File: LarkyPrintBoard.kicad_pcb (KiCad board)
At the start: 2 copper layers, 38 x 56 mm, 27 parts, among them J1 EXT1_IN, J2 EXT2_IN, J3 EXT1_OUT, J4 EXT2_OUT, J5 UART, J6 RST, J7 BOOT, J8 3V3, J9 JTAG, U1 LM1117-3.3, U2 ESP32-WROOM, U3 CBT3257A, U4 CBT3257A

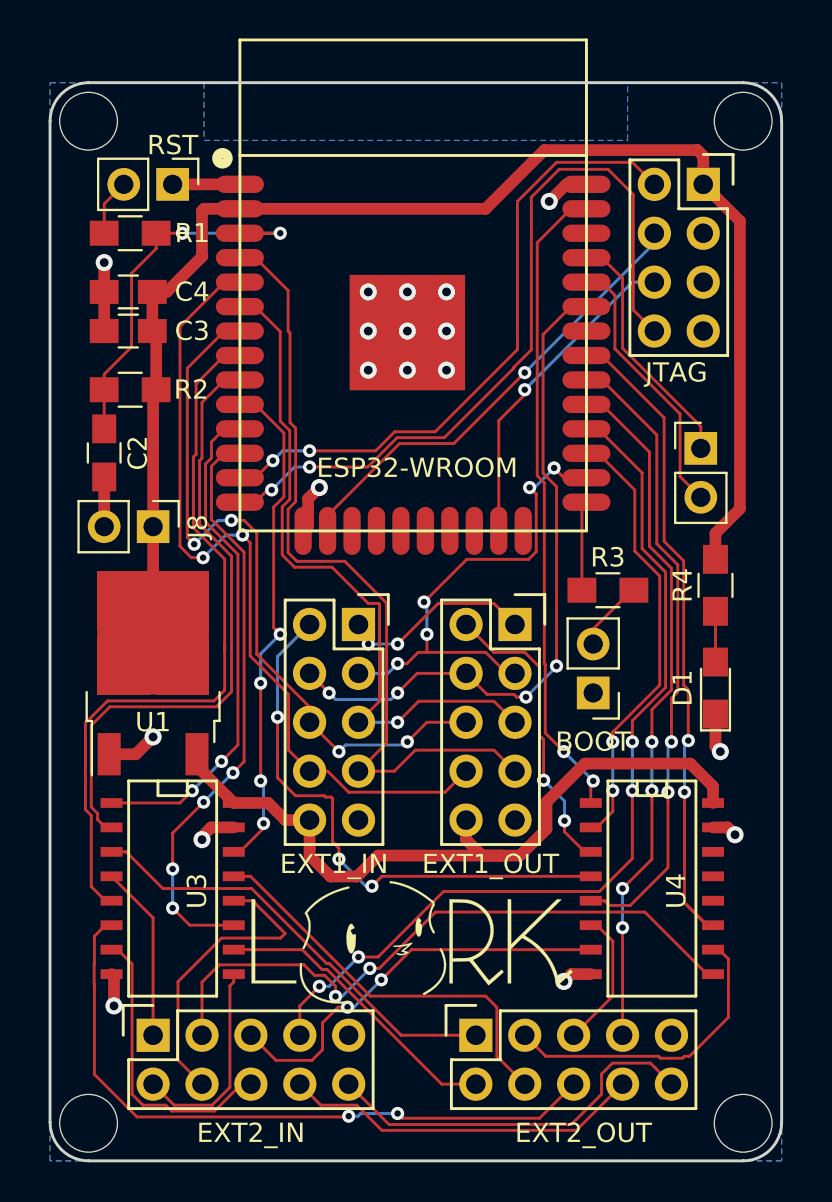
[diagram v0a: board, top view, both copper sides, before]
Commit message: Tons of changes and fixes. R1A2
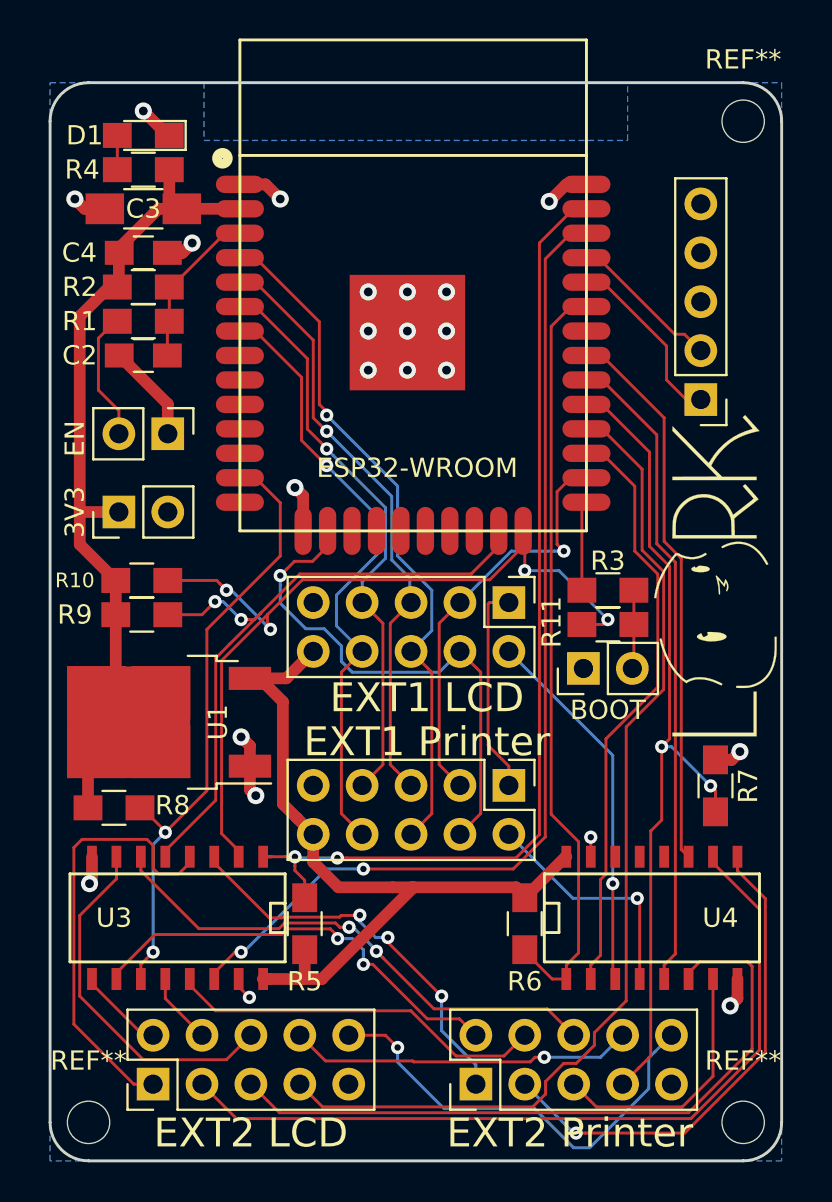
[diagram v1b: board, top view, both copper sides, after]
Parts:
- removed J9: JTAG, Socket_Strips:Socket_Strip_Straight_2x04
- removed the REF** at (146.0, 78.0)
- removed the REF** at (180.0, 78.0)
- removed the REF** at (180.0, 130.0)
- removed the REF** at (146.0, 130.0)
- removed the REF*** at (163.1, 96.5)
- added G***: LOGO, LarkyPrint:LOGO, B.Cu at (162.6, 80.8)
- added R10: 10K, Resistors_SMD:R_0805_HandSoldering, F.Cu at (148.8, 101.9)
- added R11: 680, Resistors_SMD:R_0805_HandSoldering, F.Cu at (173.0, 104.1)
- added R5: 10K, Resistors_SMD:R_0805_HandSoldering, F.Cu at (157.2, 119.7)
- added R6: 10K, Resistors_SMD:R_0805_HandSoldering, F.Cu at (168.7, 119.7)
- added R7: 10K, Resistors_SMD:R_0805_HandSoldering, F.Cu at (178.6, 112.5)
- added R8: 10K, Resistors_SMD:R_0805_HandSoldering, F.Cu at (147.3, 113.7)
- added R9: 10K, Resistors_SMD:R_0805_HandSoldering, F.Cu at (148.8, 103.6)
- added REF**: MountingHole_2.2mm_M2, Mounting_Holes:MountingHole_2.2mm_M2, F.Cu at (146.0, 130.0)
- added REF**: MountingHole_2.2mm_M2, Mounting_Holes:MountingHole_2.2mm_M2, F.Cu at (180.0, 130.0)
- added REF**: MountingHole_2.2mm_M2, Mounting_Holes:MountingHole_2.2mm_M2, F.Cu at (180.0, 78.0)
- added REF***: OSHW-Logo_5.7x6mm_SilkScreen, Symbols:OSHW-Logo_5.7x6mm_SilkScreen, B.Cu at (162.8, 97.2)
- C3: footprint Capacitors_SMD:C_0805_HandSoldering -> Capacitors_SMD:C_1206_HandSoldering
- J1: value EXT1_IN -> EXT1 Printer; footprint Socket_Strips:Socket_Strip_Straight_2x05 -> Pin_Headers:Pin_Header_Straight_2x05_Pitch2.54mm
- J2: value EXT2_IN -> EXT2 LCD; footprint Socket_Strips:Socket_Strip_Straight_2x05 -> Pin_Headers:Pin_Header_Straight_2x05_Pitch2.54mm
- J3: value EXT1_OUT -> EXT1 LCD; footprint Socket_Strips:Socket_Strip_Straight_2x05 -> Pin_Headers:Pin_Header_Straight_2x05_Pitch2.54mm
- J4: value EXT2_OUT -> EXT2 Printer; footprint Socket_Strips:Socket_Strip_Straight_2x05 -> Pin_Headers:Pin_Header_Straight_2x05_Pitch2.54mm
- J5: footprint Pin_Headers:Pin_Header_Straight_1x02_Pitch2.54mm -> Pin_Headers:Pin_Header_Straight_1x05_Pitch2.54mm
- J6: value RST -> EN
- R1, R3: value 470 -> 680
- R2: value 12K -> 10K
- R4: value 560 -> 680
- moved D1 41.3 mm to (148.8, 78.7), turned to 180 degrees
- moved R4 36.7 mm to (148.8, 80.5), turned to 0 degrees
- moved G*** 24.7 mm to (178.6, 101.6), turned to 90 degrees
- moved J6 13.0 mm to (150.1, 94.2)
- moved J1 11.4 mm to (167.8, 112.5)
- moved C3 6.40 mm to (148.8, 82.5)
- moved C2 5.45 mm to (148.8, 90.2), turned to 180 degrees
- moved R2 5.38 mm to (148.8, 86.6), turned to 0 degrees
- moved R1 4.62 mm to (148.8, 88.4)
- moved U1 2.67 mm to (150.2, 109.2), turned to 180 degrees
- moved J2 2.54 mm to (149.4, 128.0), turned to 90 degrees
- moved J4 2.54 mm to (166.1, 128.0), turned to 90 degrees
- moved J5 2.54 mm to (177.8, 92.5), turned to 180 degrees
- moved C4 2.18 mm to (148.8, 84.8), turned to 180 degrees
- moved J8 1.93 mm to (147.6, 98.3), turned to 90 degrees
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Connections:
- J5 pad 1: /ESP_TX -> /ESP_RX
- J5 pad 2: /ESP_RX -> /ESP_TX
- U2 pad 10: /ESP_SD_SS -> Net-(U2-Pad10)
- U2 pad 11: /SD_MUX_S -> Net-(U2-Pad11)
- U2 pad 12: /ESP_SPI_SCK -> Net-(U2-Pad12)
- U2 pad 13: /JTAG_TMS -> /ESP_SPI_SCK
- U2 pad 14: /JTAG_TDI -> Net-(U2-Pad14)
- U2 pad 16: /JTAG_TCK -> /LCD_RS
- U2 pad 23: /JTAG_TDO -> /ESP_SPI_MOSI
- U2 pad 24: Net-(U2-Pad24) -> /ESP_SPI_MISO
- U2 pad 33: /LCD_RS -> /ENC_MUX_S
- U2 pad 36: Net-(U2-Pad36) -> /ESP_SD_SS
- U2 pad 37: /ENC_MUX_S -> /SD_MUX_S
- U2 pad 4: /LCD6 -> /LCD5
- U2 pad 5: /LCD7 -> /LCD4
- U2 pad 6: /LCD4 -> /LCD6
- U2 pad 7: /LCD5 -> /LCD7
- U2 pad 8: /ESP_SPI_MOSI -> Net-(U2-Pad8)
- U2 pad 9: /ESP_SPI_MISO -> Net-(U2-Pad9)
- U4 pad 10: /ENC_2_O -> /ENC_2_I
- U4 pad 6: /ENC_1_O -> /ENC_1_I
- U4 pad 7: /ENC_1_I -> /ENC_1_O
- U4 pad 9: /ENC_2_I -> /ENC_2_O
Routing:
- net /JTAG_TDI: track 40.3 -> 0.00 mm, vias 2 -> 0
- net /JTAG_TMS: track 33.3 -> 0.00 mm, vias 2 -> 0
- net +3V3: track 73.4 -> 40.4 mm
- net /ESP_SD_SS: track 26.3 -> 53.1 mm, vias 4 -> 2
- net /SD_MUX_S: track 26.7 -> 51.7 mm
- net /JTAG_TCK: track 24.3 -> 0.00 mm, vias 1 -> 0
- net /JTAG_TDO: track 17.3 -> 0.00 mm, vias 1 -> 0
- net /ENC_BTN_I: track 29.1 -> 12.3 mm, vias 3 -> 1
- net /ENC_1_I: track 21.4 -> 36.8 mm, vias 2 -> 0
- net /SD_MISO_I: track 9.15 -> 23.1 mm
- net /ESP_SPI_MISO: track 32.7 -> 45.6 mm, vias 0 -> 4
- net /SD_SS_I: track 15.8 -> 3.71 mm
- net /LCD6: track 42.5 -> 30.7 mm, vias 0 -> 1
- net /EN: track 19.8 -> 8.42 mm, vias 2 -> 0
- net /ENC_2_O: track 16.3 -> 26.0 mm, vias 0 -> 1
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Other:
- rule pad_to_mask_clearance: 0.2 -> 0.0762
- board text added: "Lark R1-A2 - 09.23.2017 Copyright Greg Lincoln CC BY-NC-SA"
- board text removed: "Lark R1-A1 - 09.07.2017 Copyright Greg Lincoln CC BY-NC-SA"
